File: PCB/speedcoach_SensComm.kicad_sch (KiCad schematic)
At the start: 15 parts, among them J1 Conn_01x04_Male, J2 Conn_01x04_Male, U1 PA1010D, U2 DA14531MOD, U3 ORG1411-PM04, U4 GLCD_2.7INCH, U5 PIM456, U6 Bluefruit, U7 MB85RS256TY

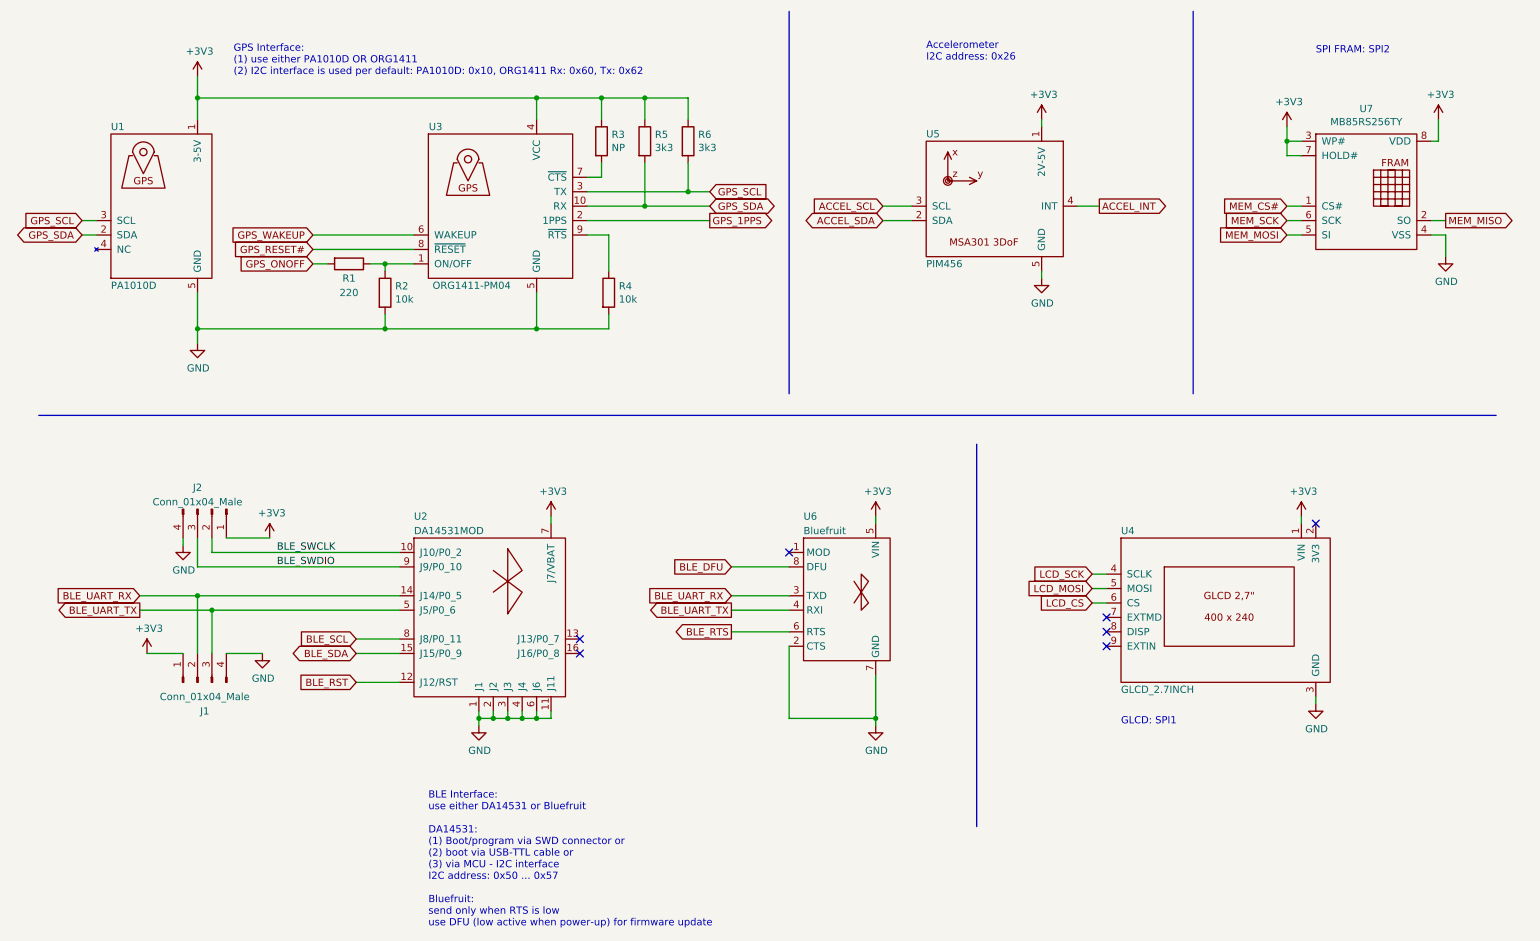
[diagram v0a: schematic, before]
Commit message: revised MCU
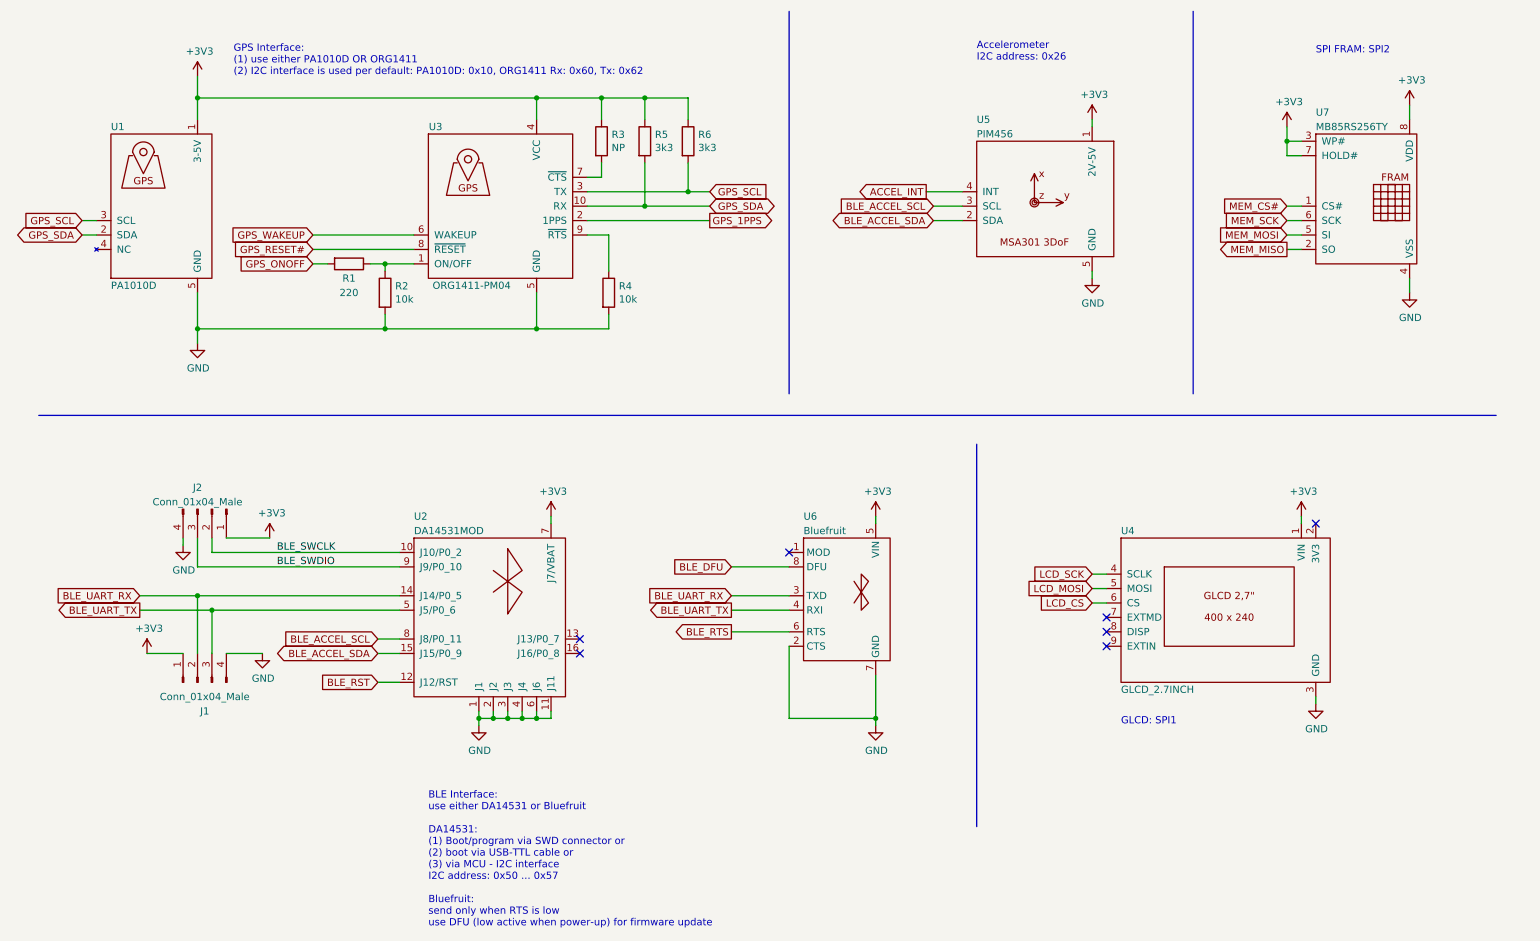
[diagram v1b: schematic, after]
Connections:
- net BLE_SCL is gone; now on net BLE_ACCEL_SCL: U2.8 (J8/P0_11)
- net BLE_SDA is gone; now on net BLE_ACCEL_SDA: U2.15 (J15/P0_9)
- net ACCEL_SCL renamed BLE_ACCEL_SCL
- net ACCEL_SDA renamed BLE_ACCEL_SDA
